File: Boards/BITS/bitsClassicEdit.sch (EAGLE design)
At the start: 34 parts, among them T1 SI1013, U1 LMR16020, X2 53398-10

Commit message: All of the changes with CAD and electronics since switching to the microclasp connectors
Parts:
- added R4: (no value), resistor:R-US_R0603
- added U$5: (no value), NR_connectors:MICROCLASP
- U$1: value MOLEX_NANOFIT_2 -> (none); device cmdLibs:MOLEX_NANOFIT_2 -> NR_connectors:MICROCLASP
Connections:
- removed net X: U$2.14/A0
- new net N$32: R4.1, U$5.P$1
- new net SWITCH_LED: R4.2, U$2.14/A0
- net GND: now also U$1.P$2, U$5.P$2; no longer U$1.P2
- net IN1: now also U$1.P$1; no longer U$1.P1
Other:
- note added: "LED Status"
- note removed: "Don't forget the oscillator"
- moved on the sheet: C11, C2, C3, C4, C5, D1, D3, L1, LED1, LED2, R1, R10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

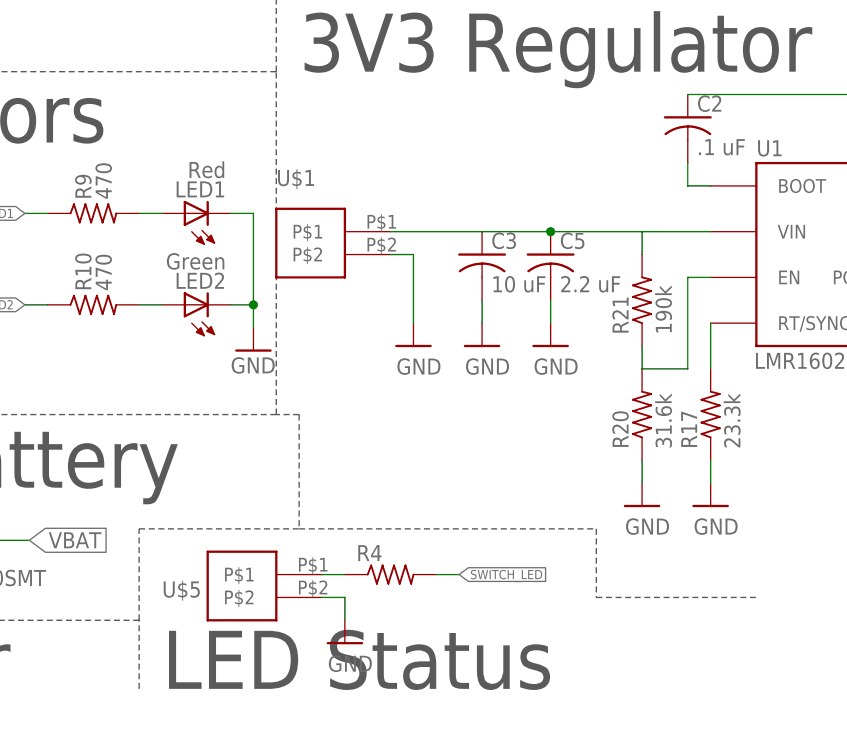
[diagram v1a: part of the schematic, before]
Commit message: fixes and design review slides
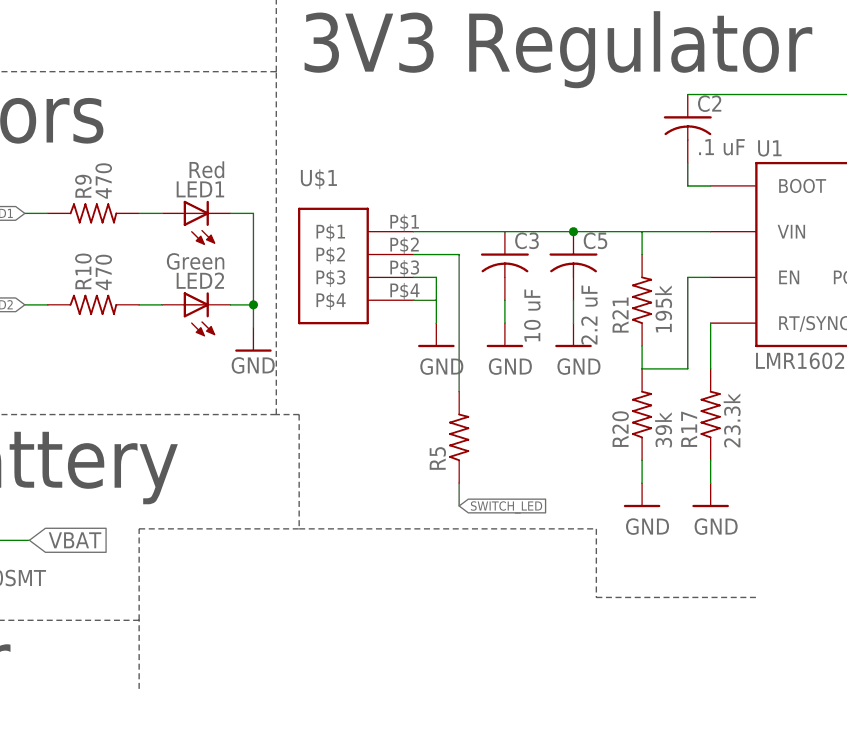
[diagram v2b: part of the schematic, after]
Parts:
- removed R4: (no value), resistor:R-US_R0603
- removed U$5: (no value), NR_connectors:MICROCLASP
- added R5: (no value), resistor:R-US_R0603
- R20: value 31.6k -> 39k
- R21: value 190k -> 195k
- U$1: value (none) -> MICROCLASP_4; device NR_connectors:MICROCLASP -> NR_connectors:MICROCLASP_4
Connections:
- removed net N$32: R4.1, U$5.P$1
- new net N$33: R5.2, U$1.P$2
- net GND: now also U$1.P$3, U$1.P$4; no longer U$1.P$2, U$5.P$2
- net SWITCH_LED: now also R5.1; no longer R4.2
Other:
- note removed: "LED Status"
- moved on the sheet: C3, C5
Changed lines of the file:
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@@
 <part name="U1" library="HASP" deviceset="LMR16020" device=""/>
 <part name="D3" library="HASP" deviceset="DO-214AC" device=""/>
-<part name="R20" library="resistor" deviceset="R-US_" device="R0603" value="31.6k"/>
-<part name="R21" library="resistor" deviceset="R-US_" device="R0603" value="190k"/>
+<part name="R20" library="resistor" deviceset="R-US_" device="R0603" value="39k"/>
+<part name="R21" library="resistor" deviceset="R-US_" device="R0603" value="195k"/>
 <part name="SUPPLY20" library="supply1" deviceset="GND" device=""/>
 <part name="T1" library="cmdLibs" deviceset="SI1013" device=""/>
@@
 <part name="+3V5" library="supply1@1" deviceset="+3V3" device=""/>
 <part name="GND6" library="supply1@1" deviceset="GND" device=""/>
-<part name="SUPPLY1" library="supply1" deviceset="GND" device=""/>
 <part name="GND5" library="supply1@1" deviceset="GND" device=""/>
 <part name="GND10" library="supply1" deviceset="GND" device=""/>
 <part name="FRAME2" library="frames" deviceset="A4L-LOC" device=""/>
 <part name="+3V6" library="supply1@1" deviceset="+3V3" device=""/>
-<part name="U$1" library="NR_connectors" deviceset="MICROCLASP" device=""/>
-<part name="U$5" library="NR_connectors" deviceset="MICROCLASP" device=""/>
-<part name="SUPPLY10" library="supply1" deviceset="GND" device=""/>
-<part name="R4" library="resistor" deviceset="R-US_" device="R0603"/>
+<part name="U$1" library="NR_connectors" deviceset="MICROCLASP_4" device=""/>
+<part name="SUPPLY1" library="supply1" deviceset="GND" device=""/>
+<part name="R5" library="resistor" deviceset="R-US_" device="R0603"/>
 </parts>
 <sheets>
@@
 <wire x1="45.72" y1="96.52" x2="45.72" y2="119.38" width="0.1524" layer="97" style="longdash"/>
 <wire x1="109.22" y1="119.38" x2="106.68" y2="119.38" width="0.1524" layer="97" style="longdash"/>
-<text x="93.98" y="88.9" size="6.4516" layer="97">LED Status</text>
 <wire x1="109.22" y1="119.38" x2="109.22" y2="106.68" width="0.1524" layer="97" style="longdash"/>
 <wire x1="91.44" y1="106.68" x2="109.22" y2="106.68" width="0.1524" layer="97" style="longdash"/>
@@
 <attribute name="VALUE" x="153.416" y="148.209" size="1.778" layer="96"/>
 </instance>
-<instance part="C3" gate="G$1" x="129.54" y="137.16" smashed="yes">
-<attribute name="NAME" x="130.556" y="137.795" size="1.778" layer="95"/>
-<attribute name="VALUE" x="130.556" y="132.969" size="1.778" layer="96"/>
+<instance part="C3" gate="G$1" x="132.08" y="137.16" smashed="yes">
+<attribute name="NAME" x="133.096" y="137.795" size="1.778" layer="95"/>
+<attribute name="VALUE" x="136.017" y="127.254" size="1.778" layer="96" rot="R90"/>
 </instance>
 <instance part="C4" gate="G$1" x="233.68" y="142.24" smashed="yes">
@@
 <attribute name="VALUE" x="234.696" y="138.049" size="1.778" layer="96"/>
 </instance>
-<instance part="C5" gate="G$1" x="137.16" y="137.16" smashed="yes">
-<attribute name="NAME" x="138.176" y="137.795" size="1.778" layer="95"/>
-<attribute name="VALUE" x="138.176" y="132.969" size="1.778" layer="96"/>
+<instance part="C5" gate="G$1" x="139.7" y="137.16" smashed="yes">
+<attribute name="NAME" x="140.716" y="137.795" size="1.778" layer="95"/>
+<attribute name="VALUE" x="142.367" y="127" size="1.778" layer="96" rot="R90"/>
 </instance>
 <instance part="C11" gate="G$1" x="243.84" y="142.24" smashed="yes">
@@
 <attribute name="VALUE" x="244.856" y="138.049" size="1.778" layer="96"/>
 </instance>
-<instance part="SUPPLY2" gate="1" x="129.54" y="127" smashed="yes">
-<attribute name="VALUE" x="127.635" y="123.825" size="1.778" layer="96"/>
-</instance>
-<instance part="SUPPLY3" gate="1" x="137.16" y="127" smashed="yes">
-<attribute name="VALUE" x="135.255" y="123.825" size="1.778" layer="96"/>
+<instance part="SUPPLY2" gate="1" x="132.08" y="127" smashed="yes">
+<attribute name="VALUE" x="130.175" y="123.825" size="1.778" layer="96"/>
+</instance>
+<instance part="SUPPLY3" gate="1" x="139.7" y="127" smashed="yes">
+<attribute name="VALUE" x="137.795" y="123.825" size="1.778" layer="96"/>
 </instance>
 <instance part="SUPPLY4" gate="1" x="154.94" y="109.22" smashed="yes">
@@
 <attribute name="VALUE" x="167.64" y="175.26" size="1.778" layer="96"/>
 </instance>
-<instance part="SUPPLY1" gate="1" x="121.92" y="127" smashed="yes">
-<attribute name="VALUE" x="120.015" y="123.825" size="1.778" layer="96"/>
-</instance>
 <instance part="GND5" gate="1" x="61.468" y="102.87" smashed="yes">
 <attribute name="VALUE" x="58.928" y="100.33" size="1.778" layer="96"/>
@@
 <attribute name="VALUE" x="248.92" y="147.32" size="1.778" layer="96"/>
 </instance>
-<instance part="U$1" gate="G$1" x="109.22" y="139.7"/>
-<instance part="U$5" gate="G$1" x="101.6" y="101.6" smashed="yes">
-<attribute name="NAME" x="93.98" y="99.06" size="1.778" layer="95"/>
-</instance>
-<instance part="SUPPLY10" gate="1" x="114.3" y="93.98" smashed="yes">
-<attribute name="VALUE" x="112.395" y="90.805" size="1.778" layer="96"/>
-</instance>
-<instance part="R4" gate="G$1" x="119.38" y="101.6"/>
+<instance part="U$1" gate="G$1" x="111.76" y="134.62"/>
+<instance part="SUPPLY1" gate="1" x="124.46" y="127" smashed="yes">
+<attribute name="VALUE" x="122.555" y="123.825" size="1.778" layer="96"/>
+</instance>
+<instance part="R5" gate="G$1" x="127" y="116.84" rot="R90"/>
 </instances>
 <busses>
@@
 <segment>
 <pinref part="C3" gate="G$1" pin="2"/>
-<wire x1="129.54" y1="129.54" x2="129.54" y2="132.08" width="0.1524" layer="91"/>
+<wire x1="132.08" y1="129.54" x2="132.08" y2="132.08" width="0.1524" layer="91"/>
 <pinref part="SUPPLY2" gate="1" pin="GND"/>
 </segment>
 <segment>
 <pinref part="C5" gate="G$1" pin="2"/>
-<wire x1="137.16" y1="132.08" x2="137.16" y2="129.54" width="0.1524" layer="91"/>
+<wire x1="139.7" y1="132.08" x2="139.7" y2="129.54" width="0.1524" layer="91"/>
 <pinref part="SUPPLY3" gate="1" pin="GND"/>
 </segment>
@@
 </segment>
 <segment>
-<pinref part="U$1" gate="G$1" pin="P$2"/>
+<pinref part="U$1" gate="G$1" pin="P$3"/>
+<wire x1="121.92" y1="134.62" x2="124.46" y2="134.62" width="0.1524" layer="91"/>
+<wire x1="124.46" y1="134.62" x2="124.46" y2="132.08" width="0.1524" layer="91"/>
+<pinref part="U$1" gate="G$1" pin="P$4"/>
+<wire x1="124.46" y1="132.08" x2="124.46" y2="129.54" width="0.1524" layer="91"/>
+<wire x1="121.92" y1="132.08" x2="124.46" y2="132.08" width="0.1524" layer="91"/>
 <pinref part="SUPPLY1" gate="1" pin="GND"/>
-<wire x1="119.38" y1="137.16" x2="121.92" y2="137.16" width="0.1524" layer="91"/>
-<wire x1="121.92" y1="137.16" x2="121.92" y2="129.54" width="0.1524" layer="91"/>
-</segment>
-<segment>
-<pinref part="U$5" gate="G$1" pin="P$2"/>
-<wire x1="111.76" y1="99.06" x2="114.3" y2="99.06" width="0.1524" layer="91"/>
-<wire x1="114.3" y1="99.06" x2="114.3" y2="96.52" width="0.1524" layer="91"/>
-<pinref part="SUPPLY10" gate="1" pin="GND"/>
 </segment>
 </net>
@@
 <wire x1="154.94" y1="139.7" x2="147.32" y2="139.7" width="0.1524" layer="91"/>
 <pinref part="C5" gate="G$1" pin="1"/>
-<junction x="137.16" y="139.7"/>
-<wire x1="147.32" y1="139.7" x2="137.16" y2="139.7" width="0.1524" layer="91"/>
-<wire x1="137.16" y1="139.7" x2="129.54" y2="139.7" width="0.1524" layer="91"/>
+<junction x="139.7" y="139.7"/>
+<wire x1="147.32" y1="139.7" x2="139.7" y2="139.7" width="0.1524" layer="91"/>
+<wire x1="139.7" y1="139.7" x2="132.08" y2="139.7" width="0.1524" layer="91"/>
 <pinref part="C3" gate="G$1" pin="1"/>
 <pinref part="U1" gate="G$1" pin="VIN"/>
 <pinref part="R21" gate="G$1" pin="2"/>
 <wire x1="147.32" y1="137.16" x2="147.32" y2="139.7" width="0.1524" layer="91"/>
-<wire x1="129.54" y1="139.7" x2="119.38" y2="139.7" width="0.1524" layer="91"/>
 <pinref part="U$1" gate="G$1" pin="P$1"/>
+<wire x1="132.08" y1="139.7" x2="121.92" y2="139.7" width="0.1524" layer="91"/>
 </segment>
 <segment>
@@
 </segment>
 <segment>
-<pinref part="R4" gate="G$1" pin="2"/>
-<wire x1="124.46" y1="101.6" x2="127" y2="101.6" width="0.1524" layer="91"/>
-<label x="127" y="101.6" size="1.016" layer="95" xref="yes"/>
+<pinref part="R5" gate="G$1" pin="1"/>
+<wire x1="127" y1="111.76" x2="127" y2="109.22" width="0.1524" layer="91"/>
+<label x="127" y="109.22" size="1.016" layer="95" xref="yes"/>
 </segment>
 </net>
@@
 </segment>
 </net>
-<net name="N$32" class="0">
-<segment>
-<pinref part="R4" gate="G$1" pin="1"/>
-<pinref part="U$5" gate="G$1" pin="P$1"/>
-<wire x1="114.3" y1="101.6" x2="111.76" y2="101.6" width="0.1524" layer="91"/>
-</segment>
-</net>
+<net name="N$33" class="0">
+<segment>
+<pinref part="U$1" gate="G$1" pin="P$2"/>
+<pinref part="R5" gate="G$1" pin="2"/>
+<wire x1="127" y1="121.92" x2="127" y2="137.16" width="0.1524" layer="91"/>
+<wire x1="127" y1="137.16" x2="121.92" y2="137.16" width="0.1524" layer="91"/>
+</segment>
+</net>
